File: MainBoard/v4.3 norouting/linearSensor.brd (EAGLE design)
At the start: 40.6 x 30.7 mm, 19 parts, among them CON1 SPI, X1 FH12-08S-1SH, X3 16MHz, X4 MINI-USB

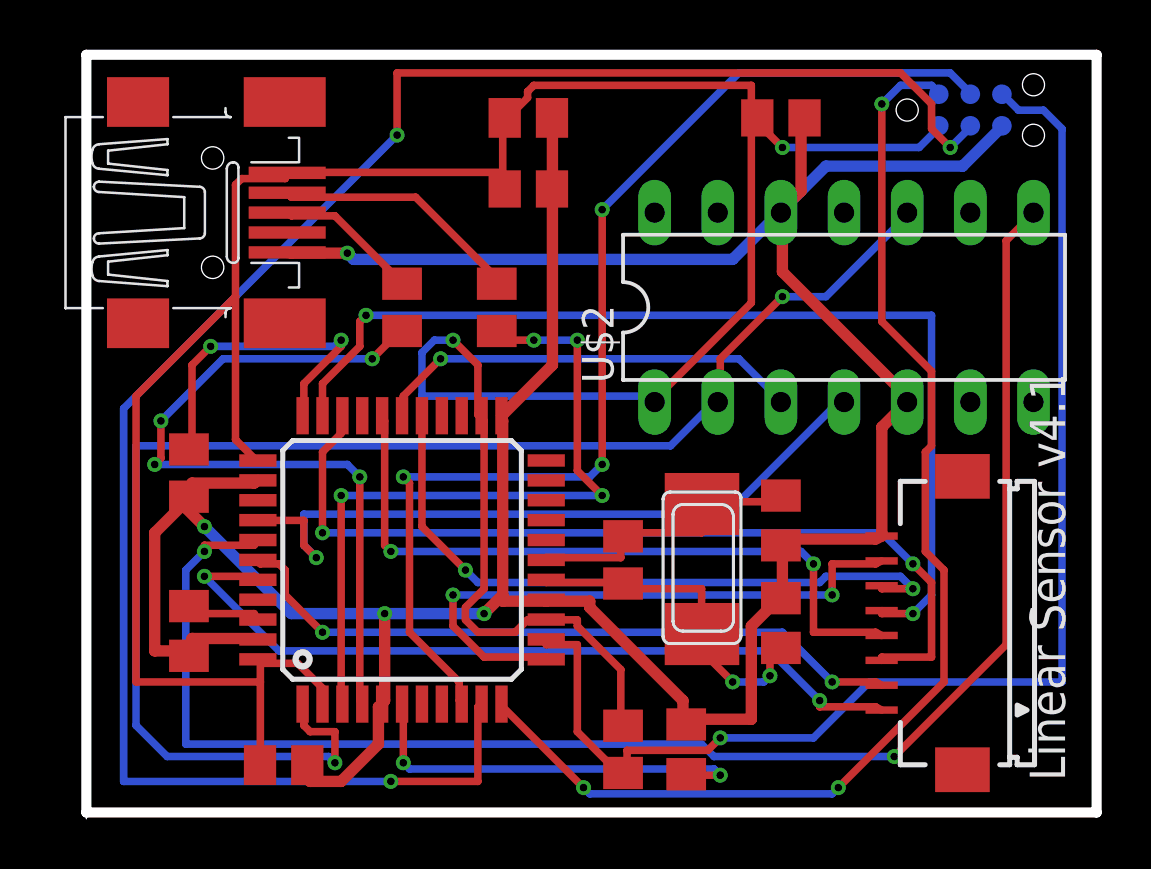
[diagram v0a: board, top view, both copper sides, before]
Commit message: Add new corrected version
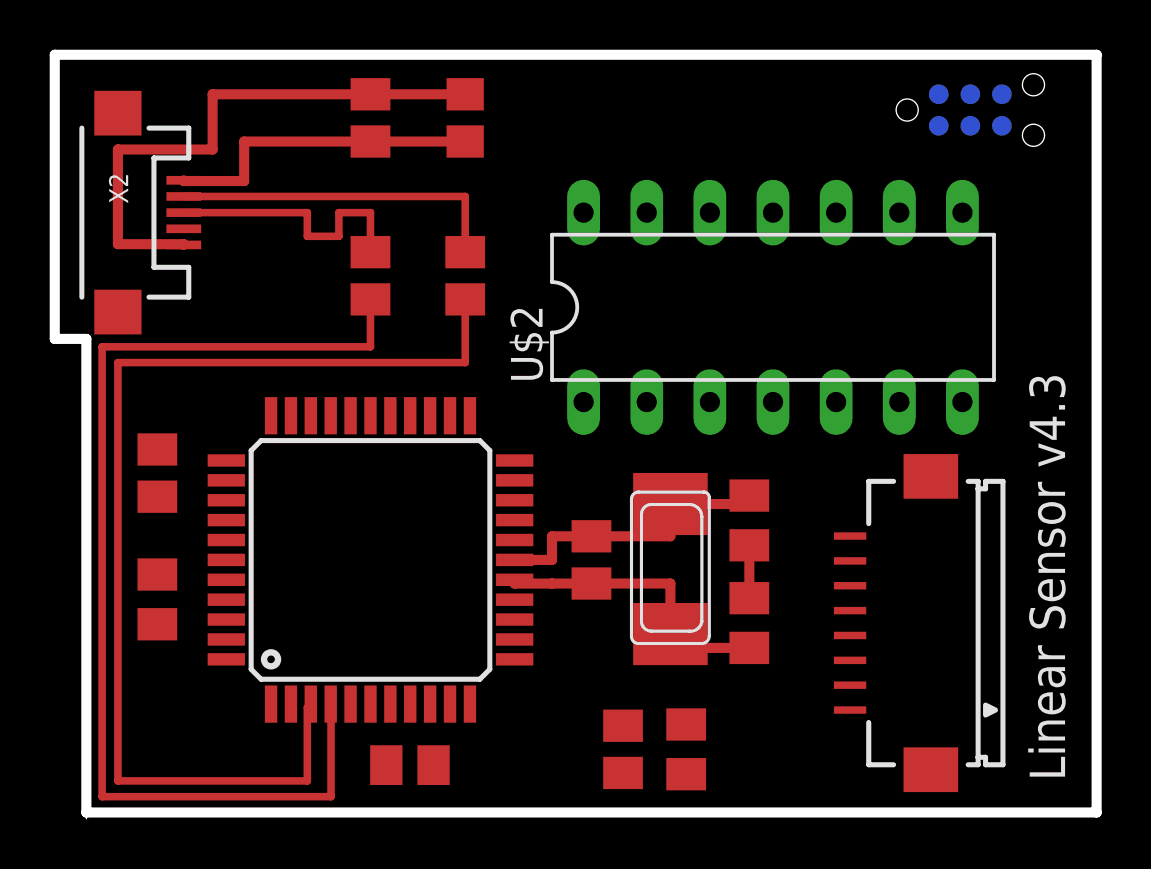
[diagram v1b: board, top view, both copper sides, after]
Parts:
- removed C7: 10uF, rcl:C0805
- removed X4: MINI-USB, con-cypressindustries:32005-201
- added X2: USB-MICROB, SparkFun:USB-MICROB
- moved C4 12.7 mm to (15.2, 27.9), turned to 270 degrees
- moved C10 6.35 mm to (11.4, 27.9), turned to 270 degrees
- moved C12 5.08 mm to (13.0, 1.91)
- moved U$2 2.86 mm to (27.6, 20.3)
- moved R31 1.80 mm to (15.2, 21.6)
- moved C11 1.80 mm to (2.86, 8.57)
- moved R24 1.80 mm to (11.4, 21.6)
- moved X1 1.27 mm to (34.0, 7.62)
- moved R3 1.27 mm to (2.86, 13.7)
- moved C2 1.27 mm to (26.7, 7.62)
- moved C8 1.27 mm to (26.7, 11.7)
- moved R13 1.27 mm to (20.3, 10.2)
- moved U$4 1.27 mm to (11.4, 10.2)
- moved X3 1.27 mm to (23.5, 9.84)
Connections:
- removed net D+USB: R24.2, X4.3
- removed net D-USB: R31.2, X4.2
- removed net VUSB: U$4.7
- new net D_USB+: R24.2, X2.D+
- new net D_USB-: R31.2, X2.D-
- net +5V/1: now also U$4.7, X2.VBUS; no longer C7.2, X4.1
- net GND: now also X2.GND; no longer C7.1, X4.5
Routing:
- net +5V/1: track 124.4 -> 12.9 mm, vias 2 -> 0
- net GND: track 135.5 -> 24.8 mm, vias 4 -> 0
- net MOSI: track 75.8 -> 0.00 mm, vias 3 -> 0
- net A2: track 63.5 -> 0.00 mm, vias 2 -> 0
- net D7*: track 59.2 -> 0.00 mm, vias 2 -> 0
- net RESET: track 52.4 -> 0.00 mm, vias 1 -> 0
- net MISO: track 48.5 -> 0.00 mm, vias 3 -> 0
- net SCK: track 46.0 -> 0.00 mm, vias 3 -> 0
- net D13*: track 41.2 -> 0.00 mm, vias 2 -> 0
- net D5*: track 35.5 -> 0.00 mm, vias 2 -> 0
- net A4: track 31.8 -> 0.00 mm, vias 2 -> 0
- net A1: track 29.1 -> 0.00 mm, vias 1 -> 0
- net D9*: track 28.3 -> 0.00 mm, vias 2 -> 0
- net A3: track 27.8 -> 0.00 mm, vias 2 -> 0
- net D6*: track 26.8 -> 0.00 mm, vias 2 -> 0
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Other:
- board size 40.6 x 30.7 mm -> 41.9 x 30.7 mm
- board text added: "Linear Sensor v4.3"
- board text removed: "Linear Sensor v4.1"
